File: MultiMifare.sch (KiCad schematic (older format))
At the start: 1 part

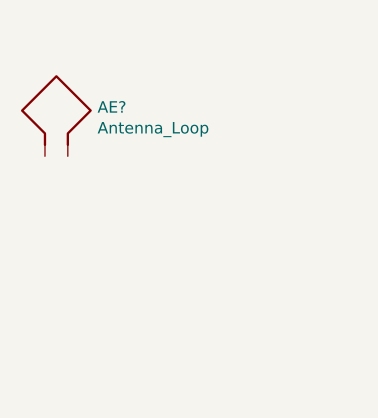
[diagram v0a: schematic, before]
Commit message: Misc
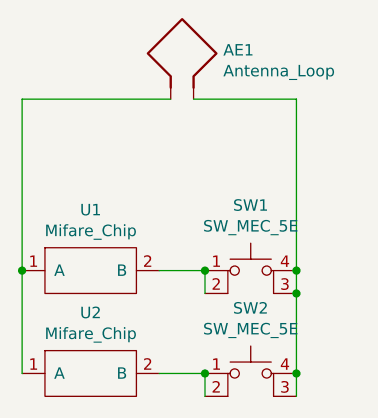
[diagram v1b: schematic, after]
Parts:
- added SW1, SW2: SW_MEC_5E, Button_Switch_SMD:SW_SPST_TL3342, symbol Switch:SW_MEC_5E
- added U1, U2: Mifare_Chip, MultiMifare:Mifare_Chip, symbol RF_Chip:Mifare_Chip
- gave numbers to parts that had none: 1
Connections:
- net at AE1.1: now also U1.1 (A), U2.1 (A)
- net at AE1.2: now also SW1.3 (K), SW1.4 (A), SW2.3 (K), SW2.4 (A)
- new net: SW1.1, SW1.2, U1.2 (B)
- new net: SW2.1, SW2.2, U2.2 (B)
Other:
- moved on the sheet: AE1
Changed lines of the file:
@@
 $EndDescr
 $Comp
-L Device:Antenna_Loop AE?
+L Device:Antenna_Loop AE1
 U 1 1 60894F4B
-P 4650 1700
-F 0 "AE?" H 4880 1714 50  0000 L CNN
-F 1 "Antenna_Loop" H 4880 1623 50  0000 L CNN
-F 2 "" H 4650 1700 50  0001 C CNN
-F 3 "~" H 4650 1700 50  0001 C CNN
-	1    4650 1700
+P 5200 1450
+F 0 "AE1" H 5430 1464 50  0000 L CNN
+F 1 "Antenna_Loop" H 5430 1373 50  0000 L CNN
+F 2 "" H 5200 1450 50  0001 C CNN
+F 3 "~" H 5200 1450 50  0001 C CNN
+	1    5200 1450
 	1    0    0    -1
 $EndComp
+$Comp
+L Switch:SW_MEC_5E SW1
+U 1 1 60997017
+P 5550 2500
+F 0 "SW1" H 5550 2885 50  0000 C CNN
+F 1 "SW_MEC_5E" H 5550 2794 50  0000 C CNN
+F 2 "Button_Switch_SMD:SW_SPST_TL3342" H 5550 2800 50  0001 C CNN
+F 3 "http://www.apem.com/int/index.php?controller=attachment&id_attachment=1371" H 5550 2800 50  0001 C CNN
+	1    5550 2500
+	1    0    0    -1
+$EndComp
+$Comp
+L RF_Chip:Mifare_Chip U1
+U 1 1 60997A4A
+P 4850 2400
+F 0 "U1" H 4850 2665 50  0000 C CNN
+F 1 "Mifare_Chip" H 4850 2574 50  0000 C CNN
+F 2 "MultiMifare:Mifare_Chip" H 4850 2550 50  0001 C CNN
+F 3 "" H 4850 2550 50  0001 C CNN
+	1    4850 2400
+	1    0    0    -1
+$EndComp
+$Comp
+L Switch:SW_MEC_5E SW2
+U 1 1 6099A78D
+P 5550 2950
+F 0 "SW2" H 5550 3335 50  0000 C CNN
+F 1 "SW_MEC_5E" H 5550 3244 50  0000 C CNN
+F 2 "Button_Switch_SMD:SW_SPST_TL3342" H 5550 3250 50  0001 C CNN
+F 3 "http://www.apem.com/int/index.php?controller=attachment&id_attachment=1371" H 5550 3250 50  0001 C CNN
+	1    5550 2950
+	1    0    0    -1
+$EndComp
+$Comp
+L RF_Chip:Mifare_Chip U2
+U 1 1 6099A793
+P 4850 2850
+F 0 "U2" H 4850 3115 50  0000 C CNN
+F 1 "Mifare_Chip" H 4850 3024 50  0000 C CNN
+F 2 "MultiMifare:Mifare_Chip" H 4850 3000 50  0001 C CNN
+F 3 "" H 4850 3000 50  0001 C CNN
+	1    4850 2850
+	1    0    0    -1
+$EndComp
+Wire Wire Line
+	5750 2950 5750 2850
+Wire Wire Line
+	5750 2850 5750 2500
+Connection ~ 5750 2850
+Wire Wire Line
+	5750 2500 5750 2400
+Connection ~ 5750 2500
+Wire Wire Line
+	5750 2400 5750 1650
+Wire Wire Line
+	5750 1650 5300 1650
+Connection ~ 5750 2400
+Wire Wire Line
+	5350 2400 5150 2400
+Wire Wire Line
+	5350 2850 5150 2850
+Wire Wire Line
+	5350 2950 5350 2850
+Connection ~ 5350 2850
+Wire Wire Line
+	5350 2500 5350 2400
+Connection ~ 5350 2400
+Wire Wire Line
+	4550 2850 4550 2400
+Wire Wire Line
+	4550 2400 4550 1650
+Wire Wire Line
+	4550 1650 5200 1650
+Connection ~ 4550 2400
 $EndSCHEMATC
